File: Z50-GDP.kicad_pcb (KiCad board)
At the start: 2 copper layers, 100 x 100 mm, 51 parts, among them J1 Z50Bus, J2 Conn_01x09, SW0 SW_Push, SW1 SW_Push, SW2 SW_Push, SW3 SW_Push, SW4 SW_Push, SW5 SW_Push, SW6 SW_Push, SW7 SW_Push, SW8 SW_DIP_x08, SW9 SW_DIP_x08, U1 74LS688, U2 74LS273, U3 74LS245, U4 74LS32

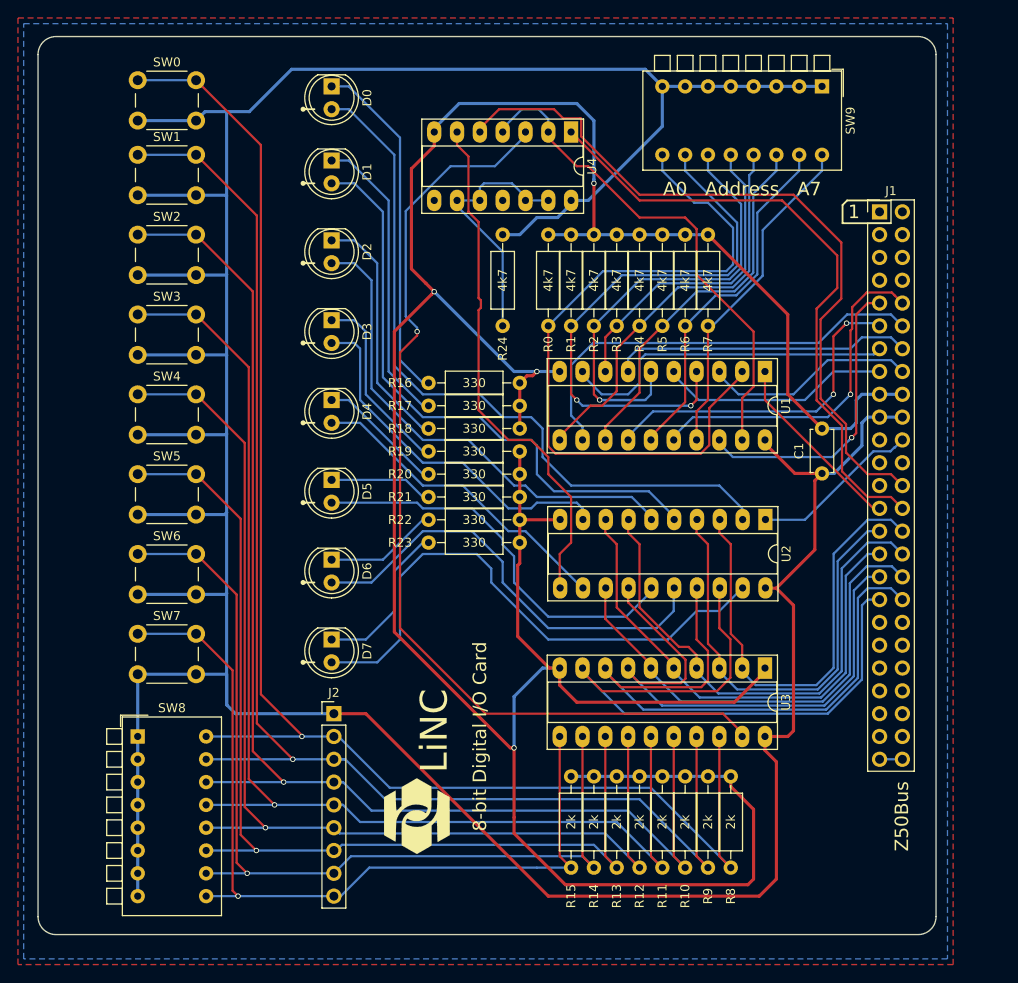
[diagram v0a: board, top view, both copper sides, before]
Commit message: Routing completed
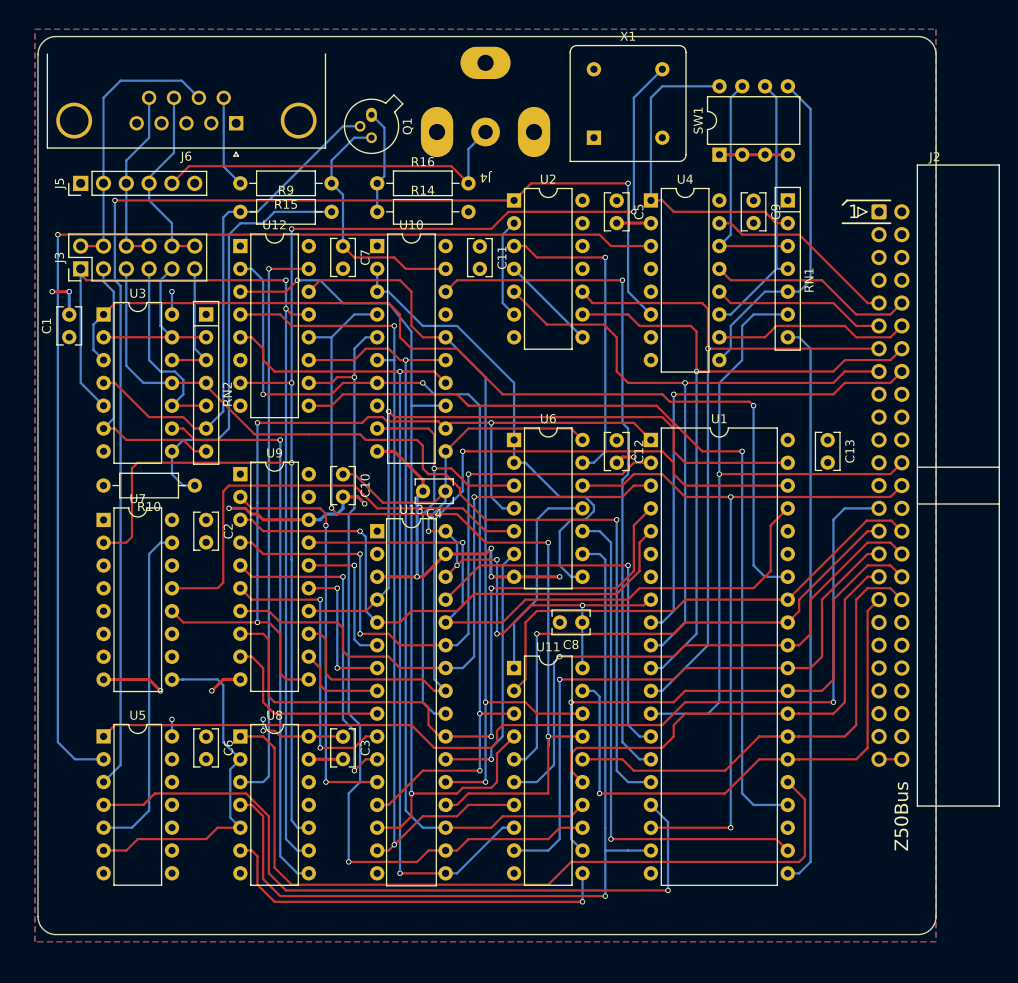
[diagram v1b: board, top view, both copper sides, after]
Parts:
- removed D0, D1, D2, D3, D4, D5, D6, D7: LED, LEDs:LED_D5.0mm
- removed G***: LOGO, LiNCLogo:LiNC_Logo
- removed J1: Z50Bus, Pin_Headers:Pin_Header_Straight_2x25_Pitch2.54mm
- removed R0, R1, R2, R24, R3, R4, R5, R6, R7: 4k7, Resistors_THT:R_Axial_DIN0207_L6.3mm_D2.5mm_P10.16mm_Horizontal
- removed R11, R12, R13, R8: 2k, Resistors_THT:R_Axial_DIN0207_L6.3mm_D2.5mm_P10.16mm_Horizontal
- removed R17, R18, R19, R20, R21, R22, R23: 330, Resistors_THT:R_Axial_DIN0207_L6.3mm_D2.5mm_P10.16mm_Horizontal
- removed SW0, SW2, SW3, SW4, SW5, SW6, SW7: SW_Push, Buttons_Switches_THT:SW_PUSH_6mm
- removed SW8, SW9: SW_DIP_x08, Buttons_Switches_THT:SW_DIP_x8_W7.62mm_Piano
- added C10: 100n, Capacitor_THT:C_Rect_L4.0mm_W2.5mm_P2.50mm, F.Cu at (137.2, 86.4)
- added C11: 100n, Capacitor_THT:C_Rect_L4.0mm_W2.5mm_P2.50mm, F.Cu at (152.4, 61.0)
- added C12: 100n, Capacitor_THT:C_Rect_L4.0mm_W2.5mm_P2.50mm, F.Cu at (167.6, 82.6)
- added C13: 100n, Capacitor_THT:C_Rect_L4.0mm_W2.5mm_P2.50mm, F.Cu at (191.1, 82.6)
- added C2: 100n, Capacitor_THT:C_Rect_L4.0mm_W2.5mm_P2.50mm, F.Cu at (121.9, 91.5)
- added C3: 100n, Capacitor_THT:C_Rect_L4.0mm_W2.5mm_P2.50mm, F.Cu at (137.2, 115.6)
- added C4: 100n, Capacitor_THT:C_Rect_L4.0mm_W2.5mm_P2.50mm, F.Cu at (148.6, 88.3)
- added C5: 100n, Capacitor_THT:C_Rect_L4.0mm_W2.5mm_P2.50mm, F.Cu at (167.6, 55.9)
- added C6: 100n, Capacitor_THT:C_Rect_L4.0mm_W2.5mm_P2.50mm, F.Cu at (121.9, 115.6)
- added C7: 100n, Capacitor_THT:C_Rect_L4.0mm_W2.5mm_P2.50mm, F.Cu at (137.2, 61.0)
- added C8: 100n, Capacitor_THT:C_Rect_L4.0mm_W2.5mm_P2.50mm, F.Cu at (163.8, 102.9)
- added C9: 100n, Capacitor_THT:C_Rect_L4.0mm_W2.5mm_P2.50mm, F.Cu at (182.9, 55.9)
- added J3: Conn_02x06_Odd_Even, Connector_PinHeader_2.54mm:PinHeader_2x06_P2.54mm_Vertical, F.Cu at (108.0, 63.5)
- added J4: Conn_Coaxial, Z50-GDP:RCA_C160_Horizontal, F.Cu at (153.0, 48.3)
- added J5: Conn_01x06, Connector_PinHeader_2.54mm:PinHeader_1x06_P2.54mm_Vertical, F.Cu at (108.0, 54.0)
- added J6: DE9_Plug_MountingHoles, Connector_Dsub:DSUB-9_Male_Horizontal_P2.77x2.84mm_EdgePinOffset4.94mm_Housed_MountingHolesOffset7.48mm, F.Cu at (125.3, 47.3)
- added Q1: BC107, Package_TO_SOT_THT:TO-18-3, F.Cu at (140.3, 46.4)
- added RN1: 1k, Resistor_THT:R_Array_SIP7, F.Cu at (186.7, 55.9)
- added RN2: 470, Resistor_THT:R_Array_SIP7, F.Cu at (121.9, 68.6)
- added U10: 74LS299, Package_DIP:DIP-20_W7.62mm, F.Cu at (141.0, 61.0)
- added U11: 74LS374, Package_DIP:DIP-20_W7.62mm, F.Cu at (156.2, 108.0)
- added U12: 74LS166, Package_DIP:DIP-16_W7.62mm, F.Cu at (125.7, 61.0)
- added U13: UM61512A, Package_DIP:DIP-32_W7.62mm, F.Cu at (141.0, 92.7)
- added U5: 74LS04, Package_DIP:DIP-14_W7.62mm, F.Cu at (110.5, 115.6)
- added U6: 74LS00, Package_DIP:DIP-14_W7.62mm, F.Cu at (156.2, 82.5)
- added U7: 74LS163, Package_DIP:DIP-16_W7.62mm, F.Cu at (110.5, 91.5)
- added U8: 74LS32, Package_DIP:DIP-14_W7.62mm, F.Cu at (125.7, 115.6)
- added U9: 74LS273, Package_DIP:DIP-20_W7.62mm, F.Cu at (125.7, 86.4)
- added X1: 14 MHz, Oscillator:Oscillator_DIP-8, F.Cu at (165.1, 48.9)
- C1: footprint Capacitors_THT:C_Disc_D4.7mm_W2.5mm_P5.00mm -> Capacitor_THT:C_Rect_L4.0mm_W2.5mm_P2.50mm
- J2: value Conn_01x09 -> Z50Bus; footprint Pin_Headers:Pin_Header_Straight_1x09_Pitch2.54mm -> Connector_IDC:IDC-Header_2x25_P2.54mm_Horizontal
- R10: value 2k -> 470; footprint Resistors_THT:R_Axial_DIN0207_L6.3mm_D2.5mm_P10.16mm_Horizontal -> Resistor_THT:R_Axial_DIN0207_L6.3mm_D2.5mm_P10.16mm_Horizontal
- R14: value 2k -> 1k; footprint Resistors_THT:R_Axial_DIN0207_L6.3mm_D2.5mm_P10.16mm_Horizontal -> Resistor_THT:R_Axial_DIN0207_L6.3mm_D2.5mm_P10.16mm_Horizontal
- R15: value 2k -> 220; footprint Resistors_THT:R_Axial_DIN0207_L6.3mm_D2.5mm_P10.16mm_Horizontal -> Resistor_THT:R_Axial_DIN0207_L6.3mm_D2.5mm_P10.16mm_Horizontal
- R16: value 330 -> 75; footprint Resistors_THT:R_Axial_DIN0207_L6.3mm_D2.5mm_P10.16mm_Horizontal -> Resistor_THT:R_Axial_DIN0207_L6.3mm_D2.5mm_P10.16mm_Horizontal
- R9: value 2k -> 150; footprint Resistors_THT:R_Axial_DIN0207_L6.3mm_D2.5mm_P10.16mm_Horizontal -> Resistor_THT:R_Axial_DIN0207_L6.3mm_D2.5mm_P10.16mm_Horizontal
- SW1: value SW_Push -> SW_DIP_x04; footprint Buttons_Switches_THT:SW_PUSH_6mm -> Package_DIP:DIP-8_W7.62mm
- U1: value 74LS688 -> EF9366; footprint Housings_DIP:DIP-20_W7.62mm_Socket_LongPads -> Package_DIP:DIP-40_W15.24mm
- U2: value 74LS273 -> 74LS08; footprint Housings_DIP:DIP-20_W7.62mm_Socket_LongPads -> Package_DIP:DIP-14_W7.62mm
- U3: value 74LS245 -> 74LS05; footprint Housings_DIP:DIP-20_W7.62mm_Socket_LongPads -> Package_DIP:DIP-14_W7.62mm
- U4: value 74LS32 -> 74LS85; footprint Housings_DIP:DIP-14_W7.62mm_Socket_LongPads -> Package_DIP:DIP-16_W7.62mm
- moved R9 89.7 mm to (125.7, 57.1), turned to 0 degrees
- moved C1 85.2 mm to (106.7, 71.1)
- moved U3 83.5 mm to (110.5, 68.6), turned to 0 degrees
- moved J2 82.5 mm to (196.8, 57.1)
- moved R15 80.7 mm to (135.9, 54.0), turned to 180 degrees
- moved R14 76.9 mm to (141.0, 57.1), turned to 0 degrees
- moved R10 69.2 mm to (120.7, 87.6), turned to 180 degrees
- moved SW1 64.8 mm to (179.1, 50.8), turned to 90 degrees
- moved U2 45.2 mm to (156.2, 55.9), turned to 0 degrees
- moved R16 27.3 mm to (141.0, 54.0), turned to 0 degrees
- moved U1 14.8 mm to (171.4, 82.6), turned to 0 degrees
- moved U4 11.7 mm to (171.4, 55.9), turned to 0 degrees
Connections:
- C1 pad 1: VCC -> +5V
- J2 pad 1: VCC -> unconnected-(J2-Pin_1-Pad1)
- J2 pad 2: Net-(J2-Pad2) -> unconnected-(J2-Pin_2-Pad2)
- J2 pad 3: Net-(J2-Pad3) -> unconnected-(J2-Pin_3-Pad3)
- J2 pad 4: Net-(J2-Pad4) -> unconnected-(J2-Pin_4-Pad4)
- J2 pad 5: Net-(J2-Pad5) -> unconnected-(J2-Pin_5-Pad5)
- J2 pad 6: Net-(J2-Pad6) -> unconnected-(J2-Pin_6-Pad6)
- J2 pad 7: Net-(J2-Pad7) -> unconnected-(J2-Pin_7-Pad7)
- J2 pad 8: Net-(J2-Pad8) -> unconnected-(J2-Pin_8-Pad8)
- J2 pad 9: Net-(J2-Pad9) -> A7
- R10 pad 1: Net-(J2-Pad4) -> Net-(R10-Pad1)
- R14 pad 1: Net-(J2-Pad8) -> Net-(Q1-E)
- R15 pad 1: Net-(J2-Pad9) -> +5V
- R15 pad 2: GND -> Net-(J6-Pad6)
- R16 pad 1: GND -> Net-(Q1-E)
- R16 pad 2: Net-(D0-Pad1) -> /BAS
- R9 pad 1: Net-(J2-Pad3) -> Net-(Q1-B)
- R9 pad 2: GND -> Net-(R10-Pad1)
- SW1 pad 1: Net-(J2-Pad3) -> GND
- SW1 pad 2: VCC -> GND
- U1 pad 1: ~{IOREQ} -> Net-(U10-Cp)
- U1 pad 10: GND -> A1
- U1 pad 11: Net-(R4-Pad1) -> A2
- U1 pad 12: A4 -> A3
- U1 pad 13: Net-(R5-Pad1) -> ~{INT}
- U1 pad 14: A5 -> Net-(U13-WR)
- U1 pad 16: A6 -> Net-(J3-Pin_5)
- U1 pad 18: A7 -> ~{WR}
- U1 pad 19: Net-(U1-Pad19) -> Net-(U1A-~{MFREE})
- U1 pad 2: Net-(R0-Pad1) -> /DAD5
- U1 pad 20: VCC -> GND
- U1 pad 3: A0 -> /DAD4
- U1 pad 4: Net-(R1-Pad1) -> /DAD3
- U1 pad 5: A1 -> /DAD6
- U1 pad 6: Net-(R2-Pad1) -> unconnected-(U1A-MSL0-Pad6)
- U1 pad 7: A2 -> unconnected-(U1A-MSL2-Pad7)
- U1 pad 8: Net-(R3-Pad1) -> +5V
- U1 pad 9: A3 -> A0
- U2 pad 1: ~{RESET} -> Net-(U4-Oa=b)
- U2 pad 10: GND -> A3
- U2 pad 11: Net-(U2-Pad11) -> unconnected-(U2-Pad11)
- U2 pad 12: Net-(D4-Pad2) -> GND
- U2 pad 13: D4 -> GND
- U2 pad 14: D5 -> +5V
- U2 pad 2: Net-(D0-Pad2) -> Net-(U2-Pad2)
- U2 pad 3: D0 -> Net-(U2-Pad3)
- U2 pad 4: D1 -> Net-(U2-Pad4)
- U2 pad 5: Net-(D1-Pad2) -> A1
- U2 pad 6: Net-(D2-Pad2) -> Net-(U2-Pad2)
- U2 pad 7: D2 -> GND
- U2 pad 8: D3 -> Net-(U2-Pad4)
- U2 pad 9: Net-(D3-Pad2) -> A2
- U3 pad 1: GND -> Net-(U1A-SYNC)
- U3 pad 10: GND -> Net-(J3-Pin_7)
- U3 pad 11: Net-(J2-Pad9) -> Net-(J3-Pin_5)
- U3 pad 12: Net-(J2-Pad8) -> Net-(J3-Pin_11)
- U3 pad 13: Net-(J2-Pad7) -> Net-(J3-Pin_9)
- U3 pad 14: Net-(J2-Pad6) -> +5V
- U3 pad 2: D0 -> Net-(J3-Pin_9)
- U3 pad 3: D1 -> Net-(U1A-SYNC)
- U3 pad 4: D2 -> Net-(Q1-B)
- U3 pad 5: D3 -> Net-(J3-Pin_1)
- U3 pad 6: D4 -> Net-(J3-Pin_3)
- U3 pad 7: D5 -> GND
- U3 pad 8: D6 -> Net-(R10-Pad1)
- U3 pad 9: D7 -> Net-(U3-Pad9)
- U4 pad 1: ~{RD} -> Net-(RN1A-R1.2)
- U4 pad 10: Net-(R24-Pad2) -> A4
- U4 pad 11: Net-(U4-Pad11) -> Net-(RN1C-R3.2)
- U4 pad 12: Net-(R24-Pad2) -> A5
- U4 pad 13: Net-(R24-Pad2) -> A6
- U4 pad 14: VCC -> Net-(RN1B-R2.2)
- U4 pad 2: Net-(U1-Pad19) -> GND
- U4 pad 3: Net-(U3-Pad19) -> Net-(U4-Ia=b)
- U4 pad 4: Net-(U1-Pad19) -> GND
- U4 pad 5: ~{WR} -> unconnected-(U4-Oa>b-Pad5)
- U4 pad 6: Net-(U2-Pad11) -> Net-(U4-Oa=b)
- U4 pad 7: GND -> unconnected-(U4-Oa<b-Pad7)
- U4 pad 8: Net-(U4-Pad8) -> GND
- U4 pad 9: Net-(R24-Pad2) -> Net-(RN1D-R4.2)
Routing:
- net VCC: track 415.2 -> 0.00 mm
- net GND: track 333.2 -> 92.5 mm, vias 4 -> 11
- net Net-(J2-Pad2): track 164.1 -> 0.00 mm, vias 1 -> 0
- net 14M: track 0.00 -> 159.1 mm, vias 0 -> 4
- net Net-(J2-Pad3): track 155.6 -> 0.00 mm, vias 1 -> 0
- net Net-(J2-Pad4): track 144.9 -> 0.00 mm, vias 1 -> 0
- net Net-(U4-Oa=b): track 0.00 -> 139.4 mm, vias 0 -> 2
- net Net-(J2-Pad5): track 134.6 -> 0.00 mm, vias 1 -> 0
- net +5V: track 0.00 -> 129.4 mm, vias 0 -> 9
- net Net-(U4-Ia=b): track 0.00 -> 129.0 mm, vias 0 -> 1
- net Net-(J2-Pad6): track 123.2 -> 0.00 mm, vias 1 -> 0
- net Net-(J2-Pad7): track 113.8 -> 0.00 mm, vias 1 -> 0
- net Net-(U3-Pad19): track 108.3 -> 0.00 mm, vias 1 -> 0
- net Net-(J3-Pin_1): track 0.00 -> 108.2 mm, vias 0 -> 2
- net Net-(U1A-SYNC): track 0.00 -> 107.3 mm, vias 0 -> 1
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- added copper zone on F.Cu, net +5V
- removed copper zone on F.Cu, net GND
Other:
- board text removed: "8-bit Digital I/O Card"
- board text removed: "A0 Address A7"
- board text removed: "LiNC"
